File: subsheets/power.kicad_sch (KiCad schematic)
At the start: 58 parts, among them J1 USB_C_Receptacle_USB2.0, U1 CP2102N, U2 MCP73871_U, U3 LP2985-3.3, U4 LTC3525-5

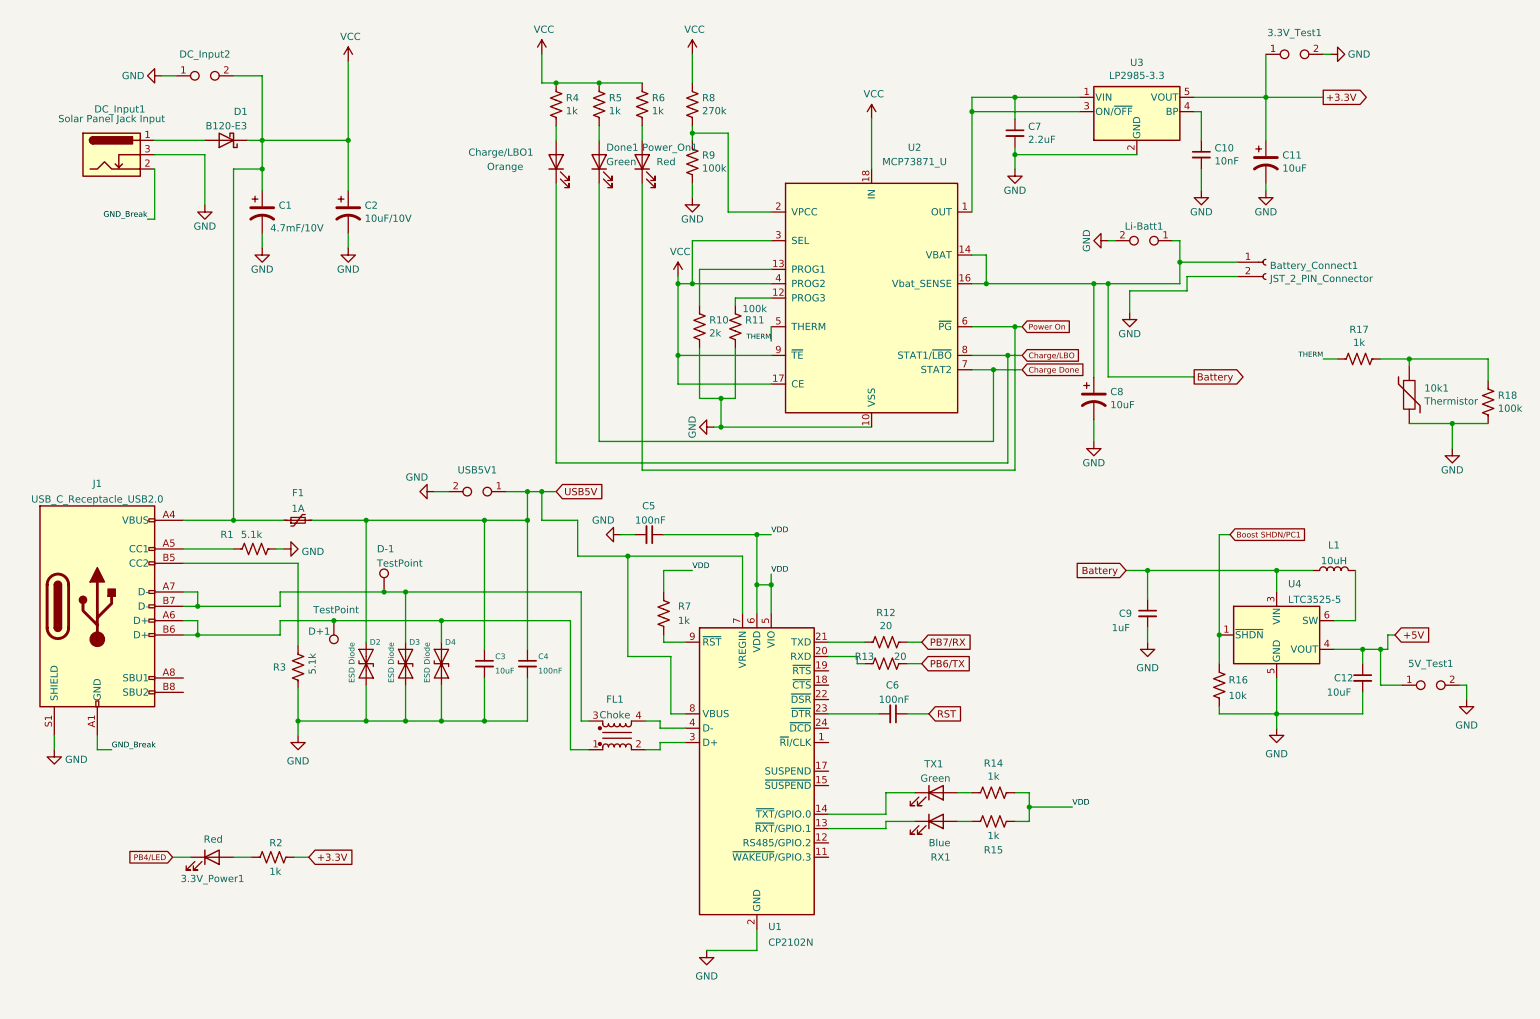
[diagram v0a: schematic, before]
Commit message: Final Schematic
-
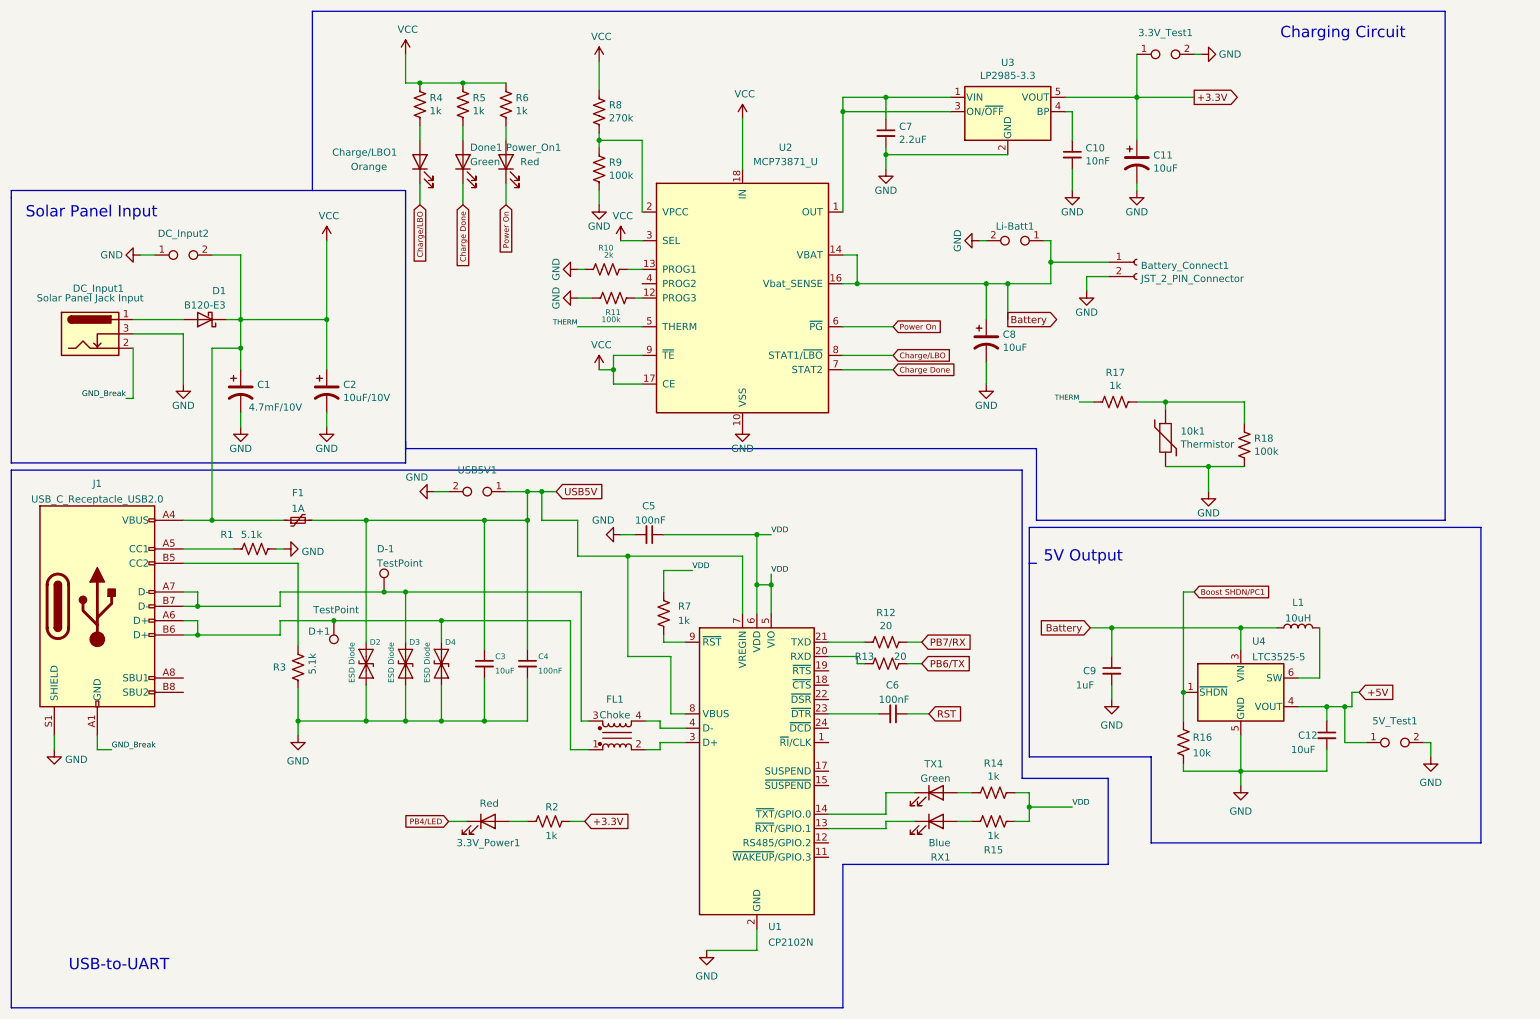
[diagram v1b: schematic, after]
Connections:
- net GND: now also R10.2, R11.2; no longer R10.1, R11.1
- net VCC: no longer U2.4 (PROG2)
- net at U2.12 (PROG3): now also R11.1; no longer R11.2
- net at U2.13 (PROG1): now also R10.1; no longer R10.2
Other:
- note added: "5V Output"
- note added: "Charging Circuit"
- note added: "Solar Panel Input"
- note added: "USB-to-UART"
- moved on the sheet: 10k1, 3.3V_Power1, 3.3V_Test1, 5V_Test1, Battery_Connect1, C1, C10, C11, C12, C2, C7, C8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
